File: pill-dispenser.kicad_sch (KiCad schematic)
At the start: 30 parts, among them J1 BAT, J2 USB_C_Receptacle_USB2.0_16P, J3 Button, J4 WS2812B, Q1 FS8205, U1 TP4056-42-ESOP8, U2 DW01A, U3 MT3608

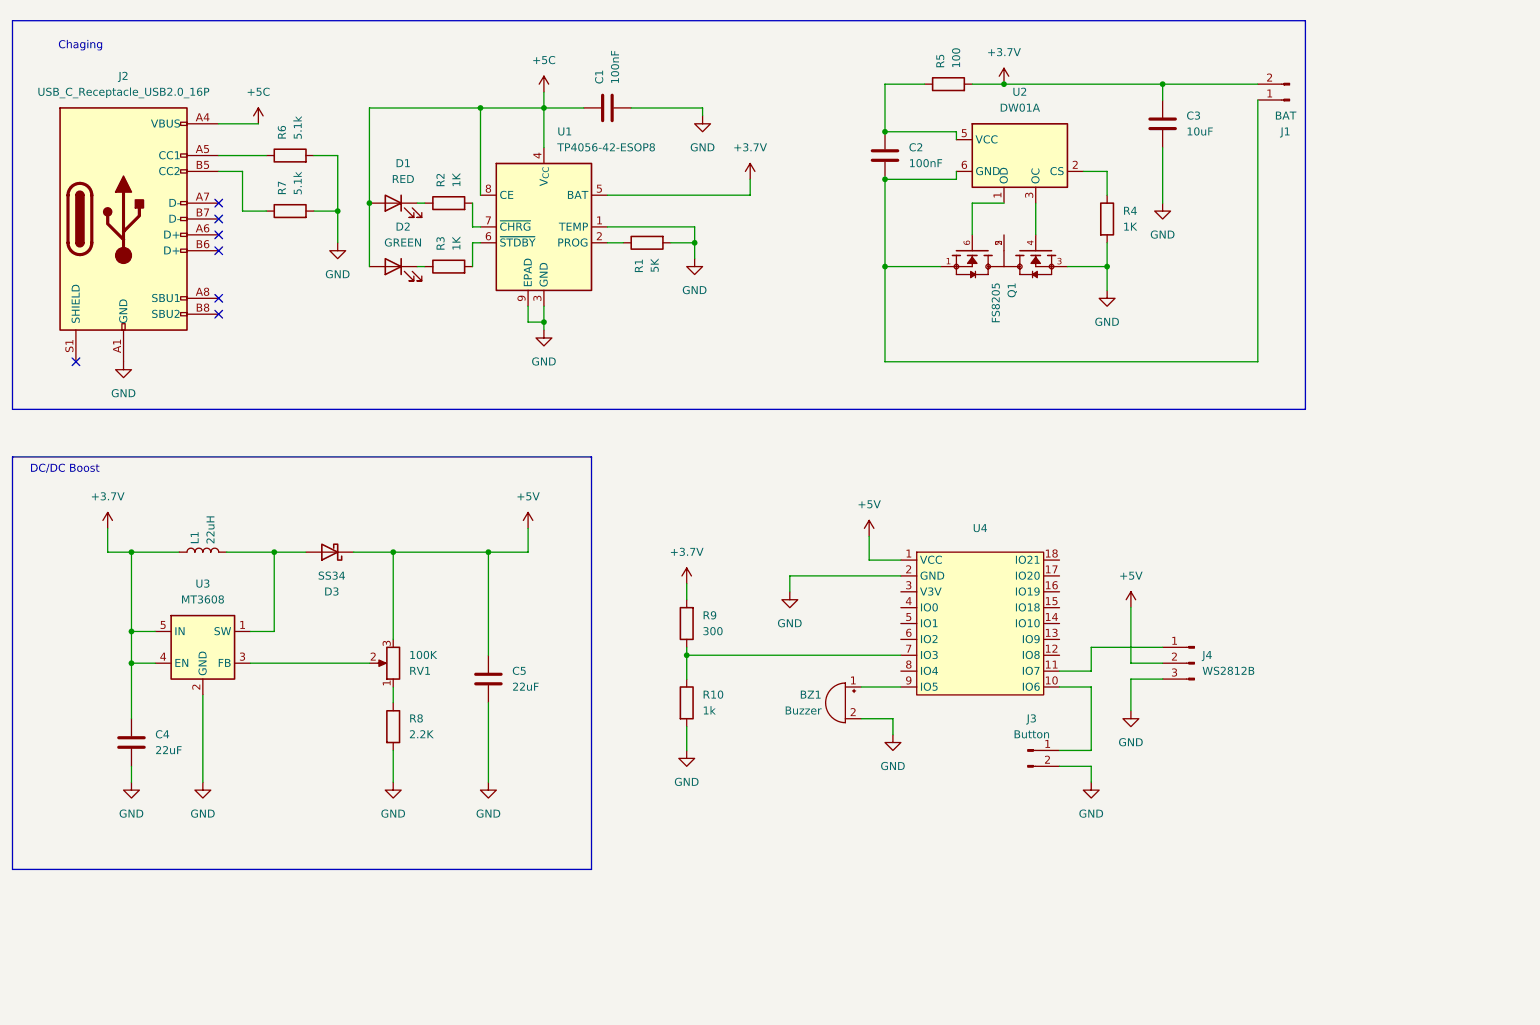
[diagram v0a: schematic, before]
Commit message: Finished schematic
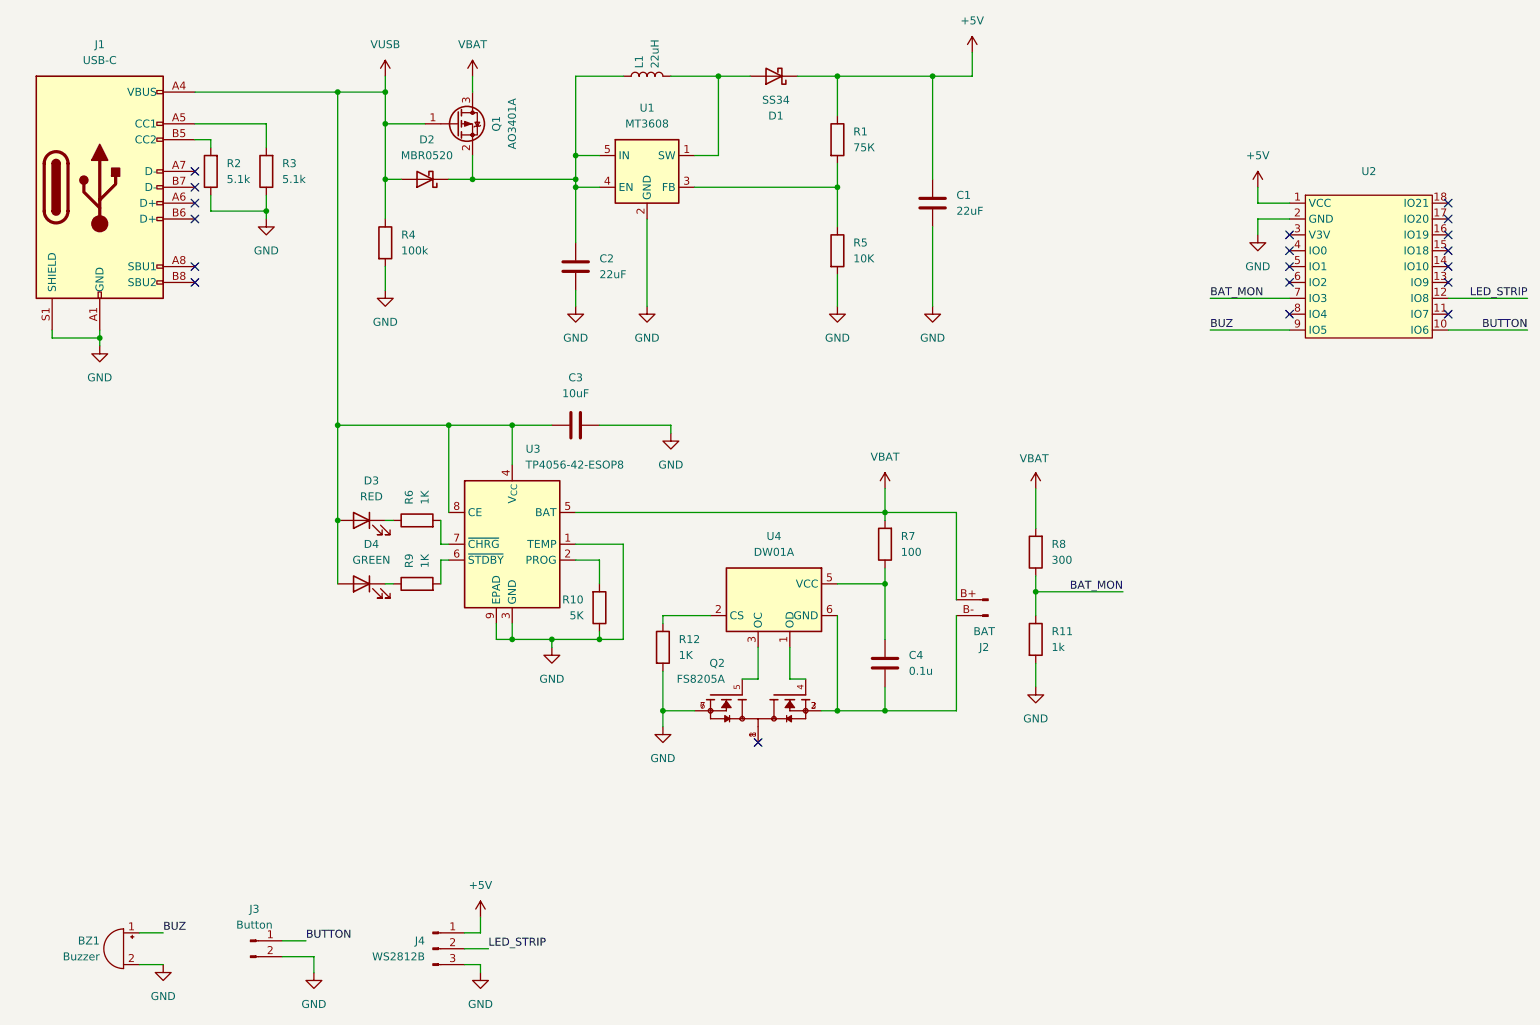
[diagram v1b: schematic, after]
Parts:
- removed C2: 100nF, symbol Device:C
- removed C3: 10uF, symbol Device:C
- removed J1: BAT, symbol Connector:Conn_01x02_Pin
- removed Q1: FS8205, FS8205:SOT95P280X145-6N, symbol FS8205:FS8205
- removed R5: 100, symbol Device:R
- removed RV1: 100K, symbol Device:R_Potentiometer
- removed U2: DW01A, Package_TO_SOT_SMD:SOT-23-6, symbol Battery_Management:DW01A
- added C4: 0.1u, symbol Device:C
- added D2: MBR0520, Diode_SMD:D_SOD-123, symbol Diode:MBR0520
- added J2: BAT, symbol Connector:Conn_01x02_Pin
- added Q1: AO3401A, Package_TO_SOT_SMD:SOT-23, symbol Transistor_FET:AO3401A
- added Q2: FS8205A, FS8205A:SOP65P640X120-8N, symbol FS8205A:FS8205A
- added R1: 75К, symbol Device:R
- added R12: 1K, symbol Device:R
- added R7: 100, symbol Device:R
- added U4: DW01A, Package_TO_SOT_SMD:SOT-23-6, symbol Battery_Management:DW01A
- BZ1: footprint (none) -> Buzzer_Beeper:Indicator_PUI_AI-1440-TWT-24V-2-R; CHIPDIP (none) -> https://www.chipdip.ru/product/hpm14a
- C3: renamed from C1; value 100nF -> 10uF
- D1: renamed from D3; CHIPDIP (none) -> https://www.chipdip.ru/product/ss34-umw
- J1: renamed from J2; value USB_C_Receptacle_USB2.0_16P -> USB-C; footprint (none) -> Connector_USB:USB_C_Plug_JAE_DX07P024AJ1; CHIPDIP (none) -> https://www.chipdip.ru/product0/8008927423
- R4: value 1K -> 100k
- R5: renamed from R8; value 2.2K -> 10K
- U3: renamed from U1; footprint Package_SO:SOIC-8-1EP_3.9x4.9mm_P1.27mm_EP2.41x3.3mm_ThermalVias -> TP4056-42-ESOP8:SOIC127P600X175-9N; CHIPDIP (none) -> https://www.chipdip.ru/product/tp4056-42-sop8-pp
- renumbered C5 to C1, C4 to C2, D1 to D3, D2 to D4, R1 to R10, R10 to R11, R7 to R2, R6 to R3, R2 to R6, R9 to R8, R3 to R9, U3 to U1, U4 to U2
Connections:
- net +5C is gone; now on net VUSB: C3.1, D3.2 (A), D4.2 (A), J1.A4 (VBUS), J1.A9 (VBUS), J1.B4 (VBUS), J1.B9 (VBUS), U3.4 (V_{CC}), U3.8 (CE)
- net +5V: now also J4.1 (Pin_1), R1.1; no longer J4.2 (Pin_2)
- net GND: now also J1.S1 (SHIELD), R10.1, R2.1, R3.1, Q2.6, Q2.7, R12.2; no longer R10.2, R2.2, R3.2
- net at U3.2 (PROG): now also R10.2; no longer R10.1
- net at J1.A5 (CC1): now also R3.2; no longer R3.1
- net at U1.3 (FB): now also R5.1, R1.2
- net at J1.B5 (CC2): now also R2.2; no longer R2.1
- net VUSB: now reaches R4.1
- net VUSB: now also D2.2 (A), Q1.1 (G)
- net BUTTON: now reaches J3.1 (Pin_1), U2.10 (IO6)
- net BUZ: now reaches BZ1.1 (+), U2.9 (IO5)
- net at U2.11 (IO7): no longer J4.1 (Pin_1)
- net LED_STRIP: now reaches U2.12 (IO8)
- net LED_STRIP: now also J4.2 (Pin_2)
- net BAT_MON: now reaches R11.1, R8.1, U2.7 (IO3)
- net +3.7V: no longer names the net of C2.1, L1.1, U1.4 (EN), U1.5 (IN)
- net +3.7V: now also D2.1 (K), Q1.2 (S); no longer R8.2, U3.5 (BAT)
- new net: Q2.1, Q2.8
- new net: C4.2, J2.B- (Pin_1), Q2.2, Q2.3, U4.6 (GND)
- new net: Q2.4, U4.1 (OD)
- new net: Q2.5, U4.3 (OC)
- new net: R12.1, U4.2 (CS)
- new net: C4.1, R7.1, U4.5 (VCC)
- new net VBAT: J2.B+ (Pin_2), Q1.3 (D), R7.2, R8.2, U3.5 (BAT)
- no-connect marks 7 -> 19
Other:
- note removed: "Chaging"
- note removed: "DC/DC Boost"
- moved on the sheet: BZ1, C1, C2, C3, D1, D3, D4, J1, J3, J4, L1, R10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
